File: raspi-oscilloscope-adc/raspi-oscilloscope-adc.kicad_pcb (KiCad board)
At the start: 2 copper layers, 80 x 50 mm, 25 parts, among them J1 Conn_Coaxial, J2 Conn_01x10_Male, J3 Conn_01x02_Male, SW1 SR10010F-0106-20F0B-C7-N-0027, U1 ECS-220B-100, U2 TLC5510INSR, U3 OPA690

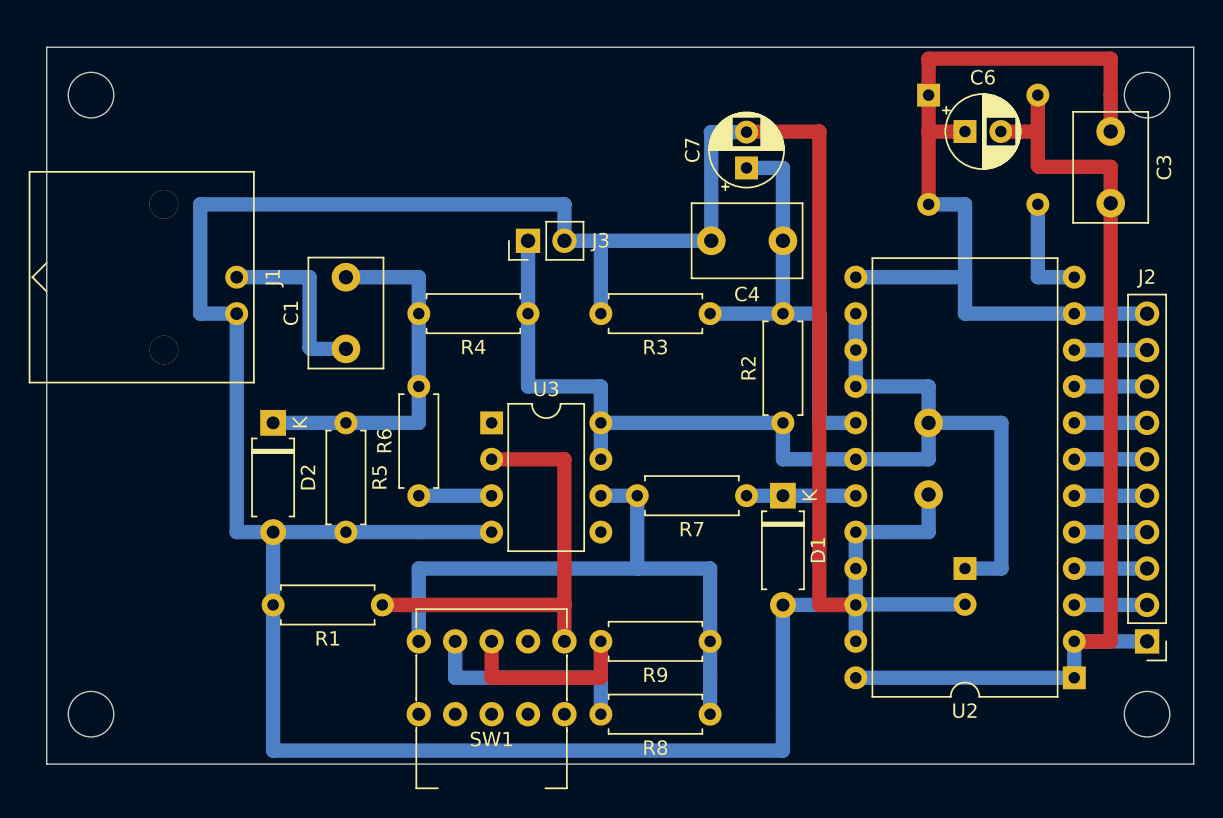
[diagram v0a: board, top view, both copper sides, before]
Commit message: Realign pcb to grid
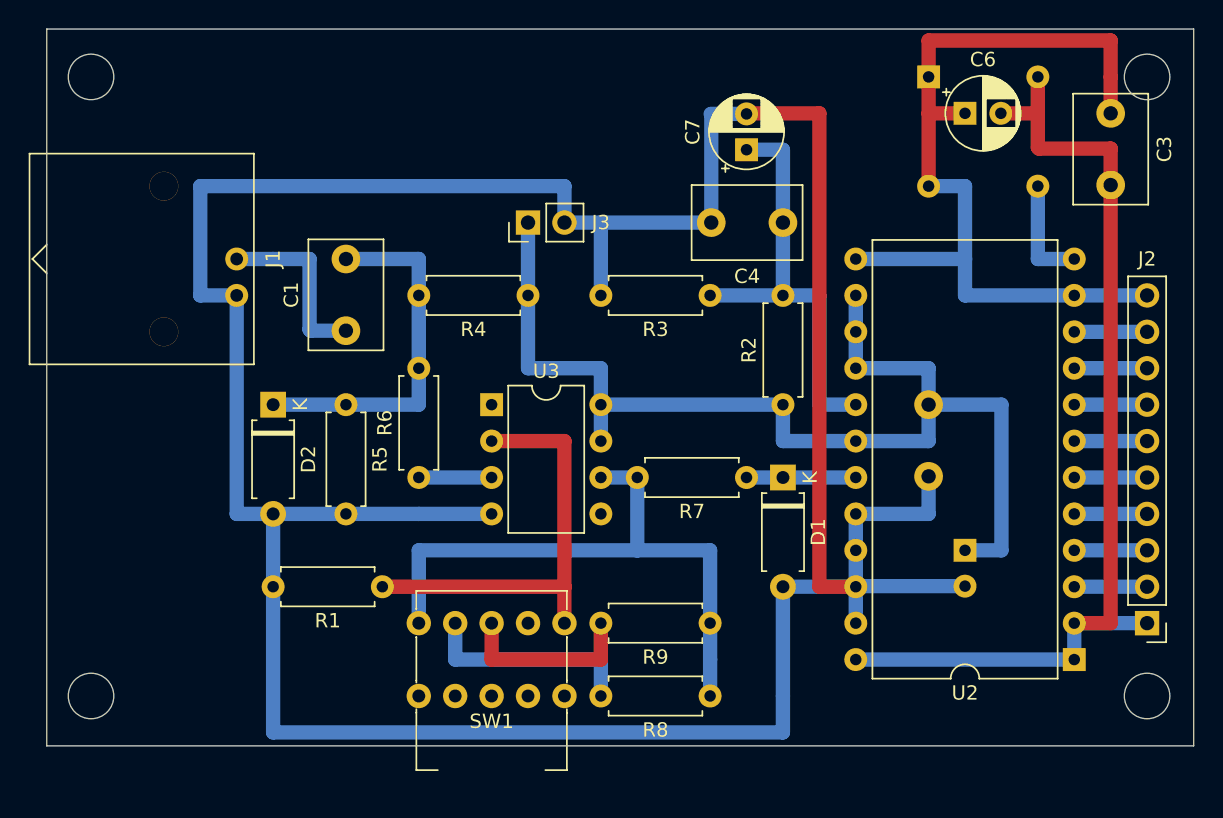
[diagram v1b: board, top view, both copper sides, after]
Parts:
- moved C2 1.27 mm to (167.6, 96.5)
- moved C4 1.27 mm to (157.5, 83.8)
- moved C7 1.27 mm to (154.9, 78.7)
- moved D1 1.27 mm to (157.5, 101.6)
- moved D2 1.27 mm to (121.9, 96.5)
- moved J3 1.27 mm to (139.7, 83.8)
- moved R2 1.27 mm to (157.5, 96.5)
- moved R5 1.27 mm to (127.0, 96.5)
- moved R6 1.27 mm to (132.1, 101.6)
- moved R7 1.27 mm to (154.9, 101.6)
- moved U1 1.27 mm to (167.6, 73.7)
- moved U3 1.27 mm to (137.2, 96.5)
- moved C1 1.27 mm to (127.0, 86.4)
- moved C3 1.27 mm to (180.3, 76.2)
- moved C5 1.27 mm to (170.2, 106.7)
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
